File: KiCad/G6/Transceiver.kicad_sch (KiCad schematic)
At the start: 4 parts, among them U1 ISL83488IBZ, U9 SN65HVD74DR

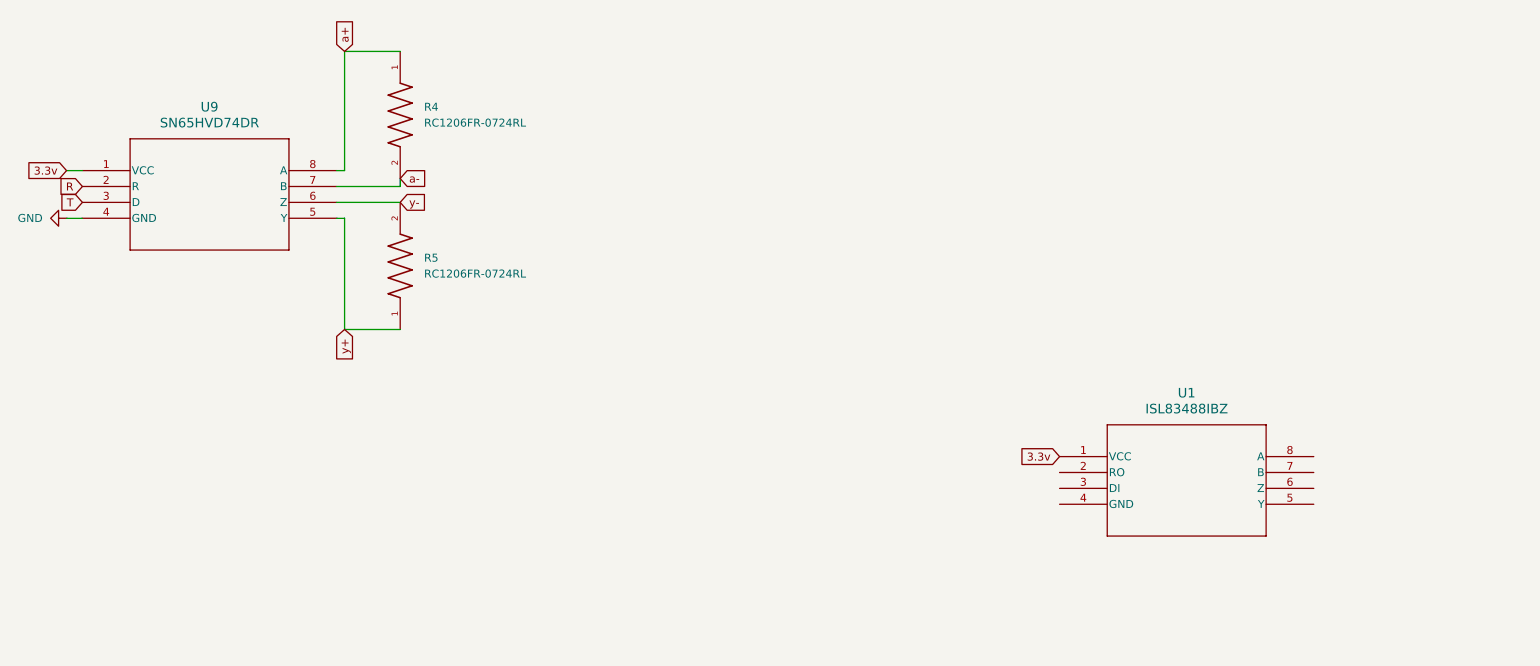
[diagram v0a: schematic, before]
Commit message: i have no idea whats going on, everything crashed and nothing will open
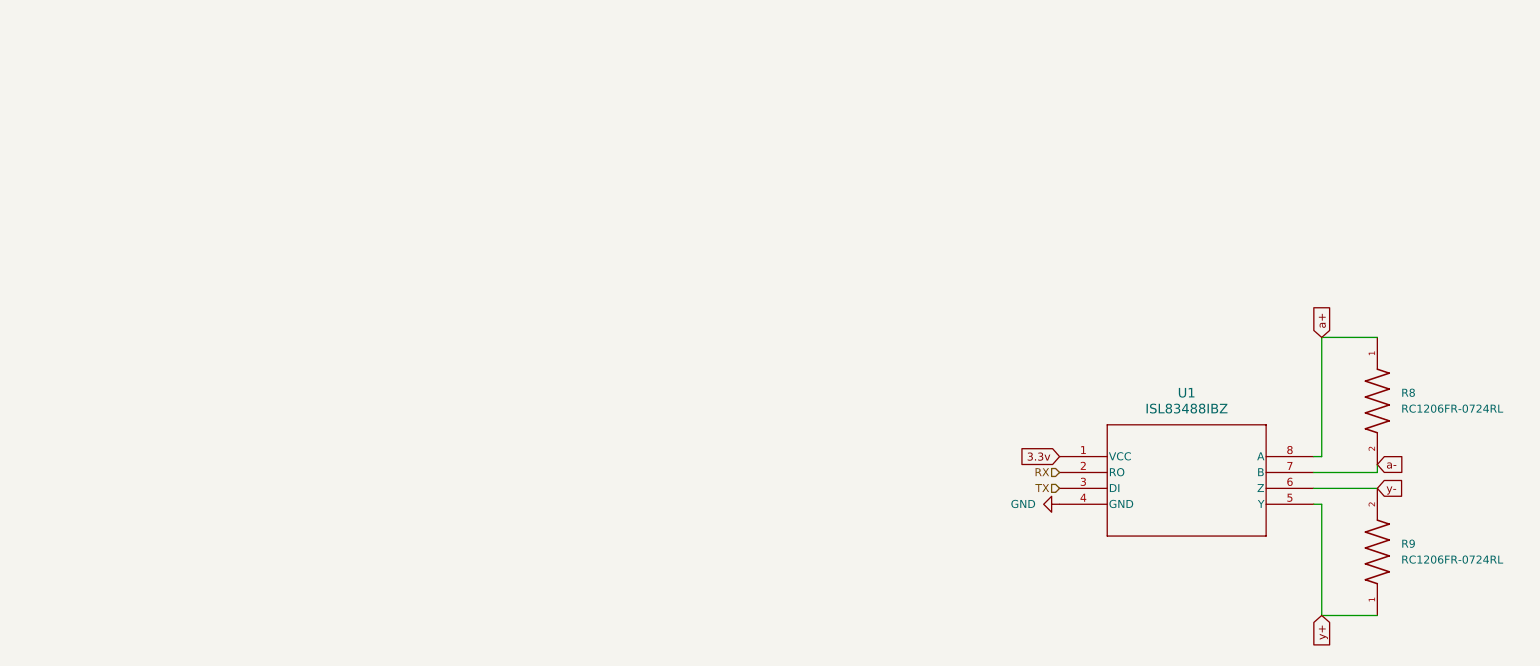
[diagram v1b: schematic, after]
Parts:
- removed R4, R5: RC1206FR-0724RL, Resistor_SMD:R_1206_3216Metric, symbol RC1206FR-0724RL:RC1206FR-0724RL
- removed U9: SN65HVD74DR, 2N65HVD74DR:D8_TEX, symbol SN65HVD74DR Transceiver:SN65HVD74DR
- added R8, R9: RC1206FR-0724RL, Resistor_SMD:R_1206_3216Metric, symbol RC1206FR-0724RL:RC1206FR-0724RL
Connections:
- net GND: now also U1.4 (GND)
- net a+: now also U1.8 (A), R8.1
- net a-: now also U1.7 (B), R8.2
- net y+: now also U1.5 (Y), R9.1
- net y-: now also U1.6 (Z), R9.2
- net RX: now reaches U1.2 (RO)
- net TX: now reaches U1.3 (DI)

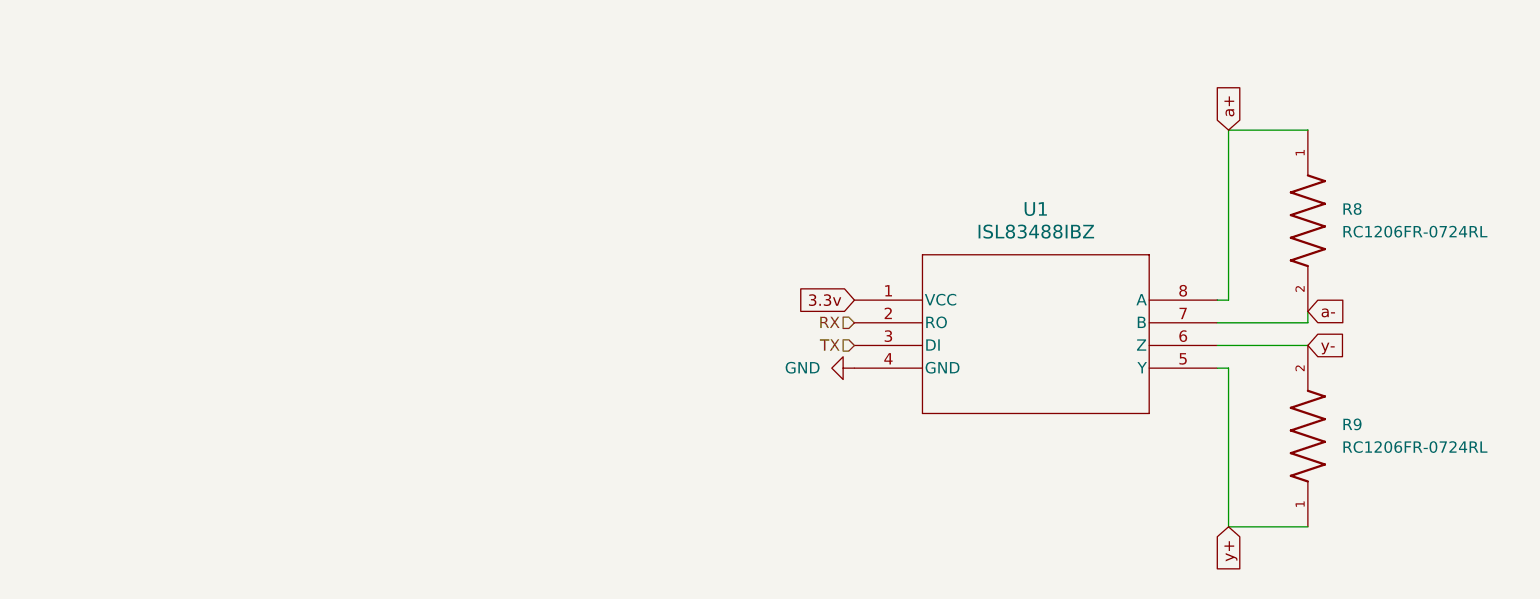
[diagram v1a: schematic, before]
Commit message: g6
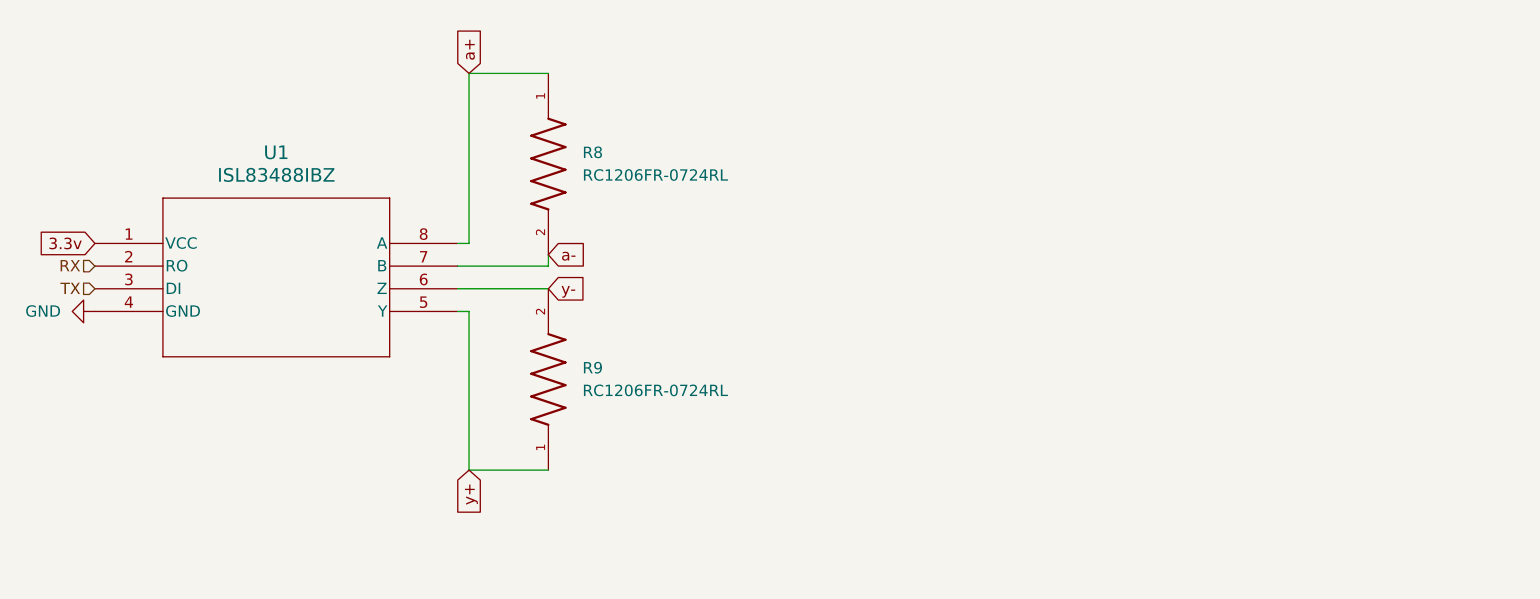
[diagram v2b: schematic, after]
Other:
- moved on the sheet: R8, R9, U1
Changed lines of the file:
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@@
 	(wire
 		(pts
-			(xy 236.22 102.87) (xy 236.22 120.65)
-		)
-		(stroke
-			(width 0)
-			(type default)
-		)
-	)
-	(wire
-		(pts
-			(xy 245.11 100.33) (xy 234.95 100.33)
-		)
-		(stroke
-			(width 0)
-			(type default)
-		)
-	)
-	(wire
-		(pts
-			(xy 245.11 97.79) (xy 234.95 97.79)
-		)
-		(stroke
-			(width 0)
-			(type default)
-		)
-	)
-	(wire
-		(pts
-			(xy 236.22 76.2) (xy 245.11 76.2)
-		)
-		(stroke
-			(width 0)
-			(type default)
-		)
-	)
-	(wire
-		(pts
-			(xy 236.22 120.65) (xy 245.11 120.65)
-		)
-		(stroke
-			(width 0)
-			(type default)
-		)
-	)
-	(wire
-		(pts
-			(xy 245.11 96.52) (xy 245.11 97.79)
-		)
-		(stroke
-			(width 0)
-			(type default)
-		)
-	)
-	(wire
-		(pts
-			(xy 236.22 102.87) (xy 234.95 102.87)
-		)
-		(stroke
-			(width 0)
-			(type default)
-		)
-	)
-	(wire
-		(pts
-			(xy 236.22 76.2) (xy 236.22 95.25)
-		)
-		(stroke
-			(width 0)
-			(type default)
-		)
-	)
-	(wire
-		(pts
-			(xy 236.22 95.25) (xy 234.95 95.25)
+			(xy 151.13 96.52) (xy 151.13 114.3)
+		)
+		(stroke
+			(width 0)
+			(type default)
+		)
+	)
+	(wire
+		(pts
+			(xy 160.02 93.98) (xy 149.86 93.98)
+		)
+		(stroke
+			(width 0)
+			(type default)
+		)
+	)
+	(wire
+		(pts
+			(xy 160.02 91.44) (xy 149.86 91.44)
+		)
+		(stroke
+			(width 0)
+			(type default)
+		)
+	)
+	(wire
+		(pts
+			(xy 151.13 69.85) (xy 160.02 69.85)
+		)
+		(stroke
+			(width 0)
+			(type default)
+		)
+	)
+	(wire
+		(pts
+			(xy 151.13 114.3) (xy 160.02 114.3)
+		)
+		(stroke
+			(width 0)
+			(type default)
+		)
+	)
+	(wire
+		(pts
+			(xy 160.02 90.17) (xy 160.02 91.44)
+		)
+		(stroke
+			(width 0)
+			(type default)
+		)
+	)
+	(wire
+		(pts
+			(xy 151.13 96.52) (xy 149.86 96.52)
+		)
+		(stroke
+			(width 0)
+			(type default)
+		)
+	)
+	(wire
+		(pts
+			(xy 151.13 69.85) (xy 151.13 88.9)
+		)
+		(stroke
+			(width 0)
+			(type default)
+		)
+	)
+	(wire
+		(pts
+			(xy 151.13 88.9) (xy 149.86 88.9)
 		)
 		(stroke
@@
 	(global_label "a-"
 		(shape input)
-		(at 245.11 96.52 0)
+		(at 160.02 90.17 0)
 		(fields_autoplaced yes)
 		(effects
@@
 		)
 		(property "Intersheetrefs" "${INTERSHEET_REFS}"
-			(at 250.8166 96.52 0)
+			(at 165.7266 90.17 0)
 			(effects
 				(font
@@
 	(global_label "3.3v"
 		(shape input)
-		(at 194.31 95.25 180)
+		(at 109.22 88.9 180)
 		(fields_autoplaced yes)
 		(effects
@@
 		)
 		(property "Intersheetrefs" "${INTERSHEET_REFS}"
-			(at 187.3334 95.25 0)
+			(at 102.2434 88.9 0)
 			(effects
 				(font
@@
 	(global_label "a+"
 		(shape input)
-		(at 236.22 76.2 90)
+		(at 151.13 69.85 90)
 		(fields_autoplaced yes)
 		(effects
@@
 		)
 		(property "Intersheetrefs" "${INTERSHEET_REFS}"
-			(at 236.22 70.4934 90)
+			(at 151.13 64.1434 90)
 			(effects
 				(font
@@
 	(global_label "y-"
 		(shape input)
-		(at 245.11 100.33 0)
+		(at 160.02 93.98 0)
 		(fields_autoplaced yes)
 		(effects
@@
 		)
 		(property "Intersheetrefs" "${INTERSHEET_REFS}"
-			(at 250.6352 100.33 0)
+			(at 165.5452 93.98 0)
 			(effects
 				(font
@@
 	(global_label "y+"
 		(shape input)
-		(at 236.22 120.65 270)
+		(at 151.13 114.3 270)
 		(fields_autoplaced yes)
 		(effects
@@
 		)
 		(property "Intersheetrefs" "${INTERSHEET_REFS}"
-			(at 236.22 126.1752 90)
+			(at 151.13 119.8252 90)
 			(effects
 				(font
@@
 	(hierarchical_label "TX"
 		(shape input)
-		(at 194.31 100.33 180)
+		(at 109.22 93.98 180)
 		(effects
 			(font
@@
 	(hierarchical_label "RX"
 		(shape input)
-		(at 194.31 97.79 180)
+		(at 109.22 91.44 180)
 		(effects
 			(font
@@
 	(symbol
 		(lib_id "RC1206FR-0724RL:RC1206FR-0724RL")
-		(at 245.11 86.36 270)
+		(at 160.02 80.01 270)
 		(unit 1)
 		(exclude_from_sim no)
@@
 		(fields_autoplaced yes)
 		(property "Reference" "R8"
-			(at 248.92 85.0899 90)
+			(at 163.83 78.7399 90)
 			(effects
 				(font
@@
 		)
 		(property "Value" "RC1206FR-0724RL"
-			(at 248.92 87.6299 90)
+			(at 163.83 81.2799 90)
 			(effects
 				(font
@@
 		)
 		(property "Footprint" "Resistor_SMD:R_1206_3216Metric"
-			(at 245.11 86.36 0)
+			(at 160.02 80.01 0)
 			(effects
 				(font
@@
 		)
 		(property "Datasheet" ""
-			(at 245.11 86.36 0)
+			(at 160.02 80.01 0)
 			(effects
 				(font
@@
 		)
 		(property "Description" ""
-			(at 245.11 86.36 0)
+			(at 160.02 80.01 0)
 			(effects
 				(font
@@
 	(symbol
 		(lib_id "RC1206FR-0724RL:RC1206FR-0724RL")
-		(at 245.11 110.49 90)
+		(at 160.02 104.14 90)
 		(unit 1)
 		(exclude_from_sim no)
@@
 		(fields_autoplaced yes)
 		(property "Reference" "R9"
-			(at 248.92 109.2199 90)
+			(at 163.83 102.8699 90)
 			(effects
 				(font
@@
 		)
 		(property "Value" "RC1206FR-0724RL"
-			(at 248.92 111.7599 90)
+			(at 163.83 105.4099 90)
 			(effects
 				(font
@@
 		)
 		(property "Footprint" "Resistor_SMD:R_1206_3216Metric"
-			(at 245.11 110.49 0)
+			(at 160.02 104.14 0)
 			(effects
 				(font
@@
 		)
 		(property "Datasheet" ""
-			(at 245.11 110.49 0)
+			(at 160.02 104.14 0)
 			(effects
 				(font
@@
 		)
 		(property "Description" ""
-			(at 245.11 110.49 0)
+			(at 160.02 104.14 0)
 			(effects
 				(font
@@
 	(symbol
 		(lib_id "ISL83488IBZ:ISL83488IBZ")
-		(at 194.31 95.25 0)
+		(at 109.22 88.9 0)
 		(unit 1)
 		(exclude_from_sim no)
@@
 		(fields_autoplaced yes)
 		(property "Reference" "U1"
-			(at 214.63 85.09 0)
+			(at 129.54 78.74 0)
 			(effects
 				(font
@@
 		)
 		(property "Value" "ISL83488IBZ"
-			(at 214.63 87.63 0)
+			(at 129.54 81.28 0)
 			(effects
 				(font
@@
 		)
 		(property "Footprint" "CC0603KRXQRQBB104:SOIC8_4X5_INR"
-			(at 194.31 95.25 0)
+			(at 109.22 88.9 0)
 			(effects
 				(font
@@
 		)
 		(property "Datasheet" "ISL83488IBZ"
-			(at 194.31 95.25 0)
+			(at 109.22 88.9 0)
 			(effects
 				(font
@@
 		)
 		(property "Description" ""
-			(at 194.31 95.25 0)
+			(at 109.22 88.9 0)
 			(effects
 				(font
@@
 	(symbol
 		(lib_id "power:GND")
-		(at 194.31 102.87 270)
+		(at 109.22 96.52 270)
 		(unit 1)
 		(exclude_from_sim no)
@@
 		(fields_autoplaced yes)
 		(property "Reference" "#PWR052"
-			(at 187.96 102.87 0)
+			(at 102.87 96.52 0)
 			(effects
 				(font
@@
 		)
 		(property "Value" "GND"
-			(at 190.5 102.8699 90)
+			(at 105.41 96.5199 90)
 			(effects
 				(font
@@
 		)
 		(property "Footprint" ""
-			(at 194.31 102.87 0)
+			(at 109.22 96.52 0)
 			(effects
 				(font
@@
 		)
 		(property "Datasheet" ""
-			(at 194.31 102.87 0)
+			(at 109.22 96.52 0)
 			(effects
 				(font
@@
 		)
 		(property "Description" "Power symbol creates a global label with name \"GND\" , ground"
-			(at 194.31 102.87 0)
-			(effects
-				(font
+			(at 109.22 96.52 0)
+			(effects
+				(font
